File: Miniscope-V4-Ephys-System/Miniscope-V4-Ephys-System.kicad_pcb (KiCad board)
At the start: 4 copper layers, 58.8 x 47 mm, 150 parts, among them J1 34 Circuit Slimslack Connector, J10 Conn_01x01, J11 Conn_01x01, J12 Conn_01x01, J13 Conn_01x01, J14 Conn_01x05, J15 Conn_01x01, J16 Conn_01x01, J17 Conn_01x01, J18 Conn_01x01, J19 Conn_01x01, J2 Conn_01x01, J20 Conn_01x01, J21 Conn_01x01, J22 Conn_01x01, J23 Conn_01x01, J24 Conn_01x01, J25 Conn_01x01, J26 Conn_01x01, J27 Conn_01x01, J28 Conn_01x01, J3 Conn_01x01, J4 Conn_01x01, J5 Conn_01x01, J6 Conn_01x01, J7 Conn_01x01, J8 Conn_01x01, J9 Conn_01x01, Q1 MMBT3904LP-7B, U1 RHD2132, U2 TXB0304RUT, U3 MCP1711T-30I/5X, U4 ATSAME70N21A-CN, U5 MCP1711T-18I/5X, Y1 SMD_CRYSTAL

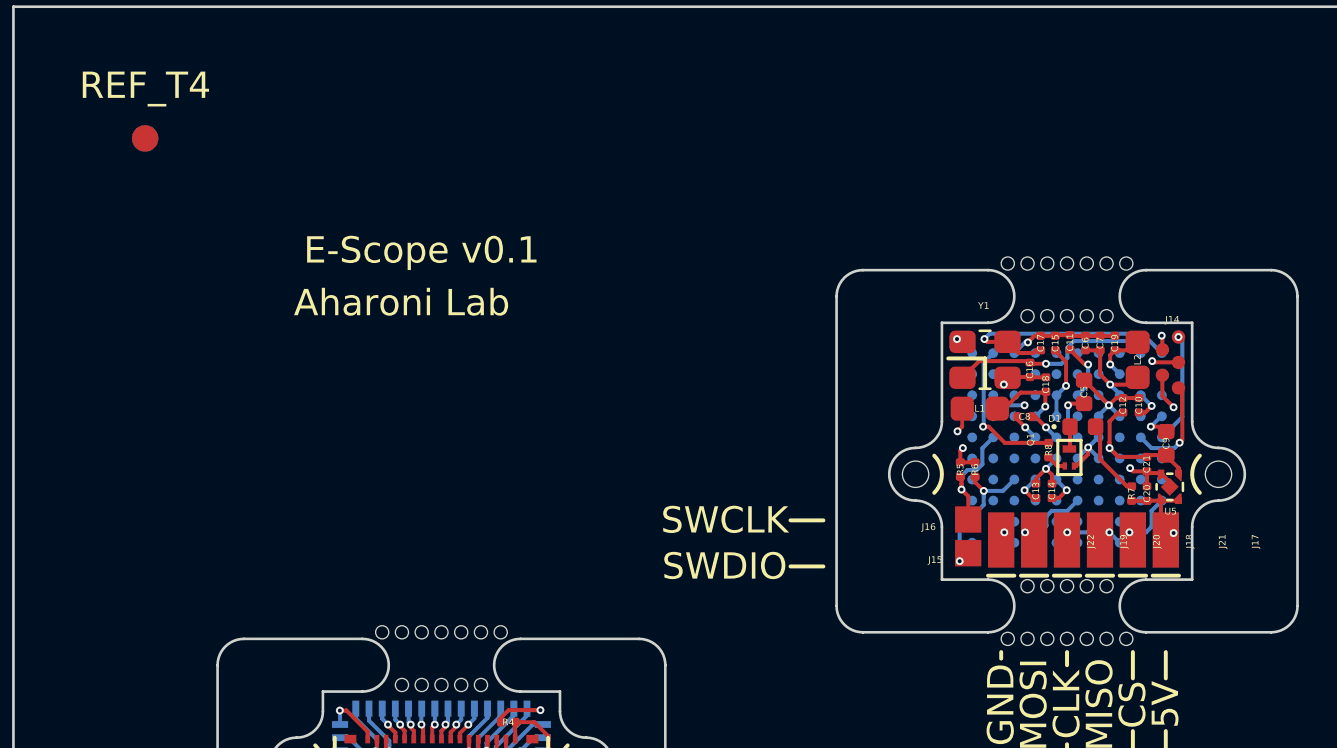
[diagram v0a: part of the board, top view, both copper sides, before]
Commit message: Add files via upload
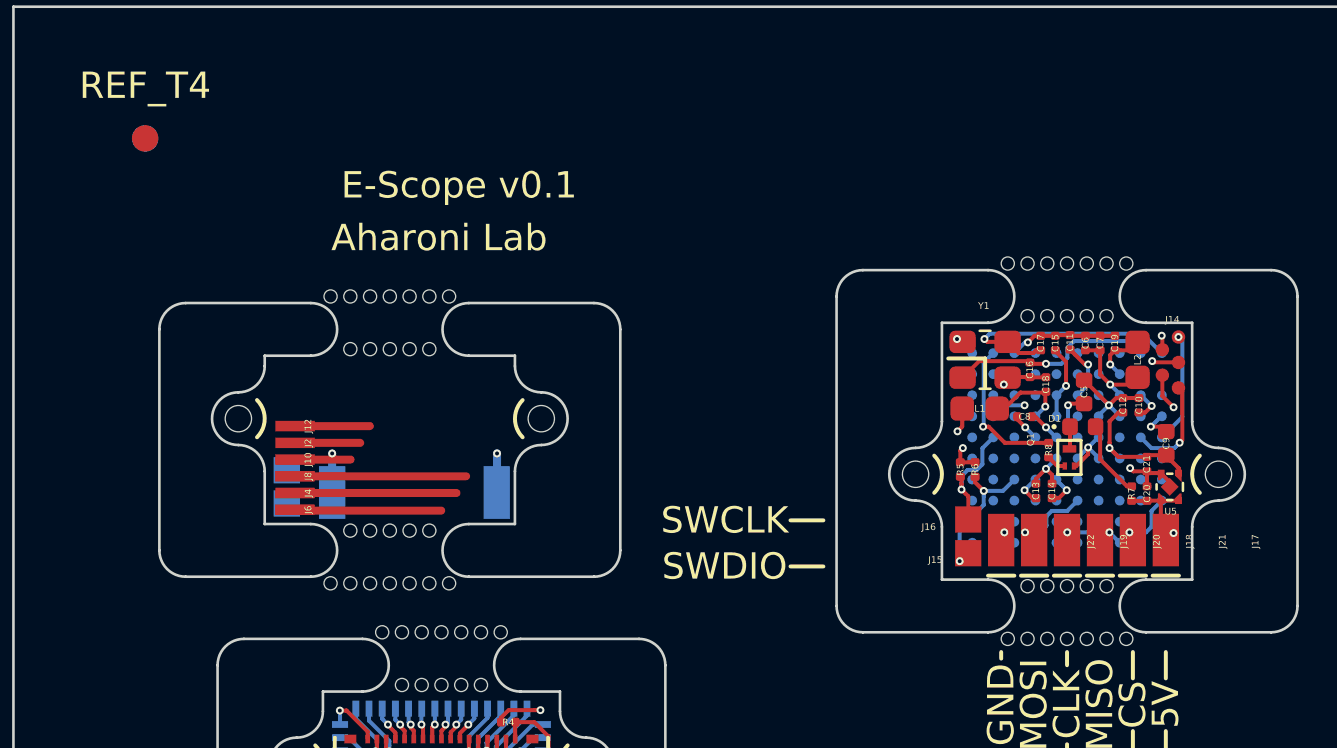
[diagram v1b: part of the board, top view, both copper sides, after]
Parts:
- added HOLE: Conn_1x1_700_Circular_Pad, .Connector:Conn_1x1_700_Circular_Pad, F.Cu at (107.8, 119.9)
- added HOLE: Conn_1x1_700_Circular_Pad, .Connector:Conn_1x1_700_Circular_Pad, F.Cu at (110.8, 111.0)
- added HOLE: Conn_1x1_700_Circular_Pad, .Connector:Conn_1x1_700_Circular_Pad, F.Cu at (110.0, 113.0)
- added HOLE: Conn_1x1_700_Circular_Pad, .Connector:Conn_1x1_700_Circular_Pad, F.Cu at (109.3, 113.0)
- added HOLE: Conn_1x1_700_Circular_Pad, .Connector:Conn_1x1_700_Circular_Pad, F.Cu at (109.3, 111.0)
- added HOLE: Conn_1x1_700_Circular_Pad, .Connector:Conn_1x1_700_Circular_Pad, F.Cu at (107.8, 111.0)
- added HOLE: Conn_1x1_700_Circular_Pad, .Connector:Conn_1x1_700_Circular_Pad, F.Cu at (108.5, 111.0)
- added HOLE: Conn_1x1_700_Circular_Pad, .Connector:Conn_1x1_700_Circular_Pad, F.Cu at (107.8, 113.0)
- added HOLE: Conn_1x1_700_Circular_Pad, .Connector:Conn_1x1_700_Circular_Pad, F.Cu at (110.8, 113.0)
- added HOLE: Conn_1x1_700_Circular_Pad, .Connector:Conn_1x1_700_Circular_Pad, F.Cu at (110.0, 111.0)
- added HOLE: Conn_1x1_700_Circular_Pad, .Connector:Conn_1x1_700_Circular_Pad, F.Cu at (108.5, 113.0)
- added HOLE: Conn_1x1_700_Circular_Pad, .Connector:Conn_1x1_700_Circular_Pad, F.Cu at (108.5, 121.9)
- added HOLE: Conn_1x1_700_Circular_Pad, .Connector:Conn_1x1_700_Circular_Pad, F.Cu at (107.8, 121.9)
- added HOLE: Conn_1x1_700_Circular_Pad, .Connector:Conn_1x1_700_Circular_Pad, F.Cu at (108.5, 119.9)
- added HOLE: Conn_1x1_700_Circular_Pad, .Connector:Conn_1x1_700_Circular_Pad, F.Cu at (109.3, 119.9)
- added HOLE: Conn_1x1_700_Circular_Pad, .Connector:Conn_1x1_700_Circular_Pad, F.Cu at (109.3, 121.9)
- added HOLE: Conn_1x1_700_Circular_Pad, .Connector:Conn_1x1_700_Circular_Pad, F.Cu at (110.8, 121.9)
- added HOLE: Conn_1x1_700_Circular_Pad, .Connector:Conn_1x1_700_Circular_Pad, F.Cu at (110.0, 121.9)
- added HOLE: Conn_1x1_700_Circular_Pad, .Connector:Conn_1x1_700_Circular_Pad, F.Cu at (110.8, 119.9)
- added HOLE: Conn_1x1_700_Circular_Pad, .Connector:Conn_1x1_700_Circular_Pad, F.Cu at (110.0, 119.9)
- added HOLE: Conn_1x1_700_Circular_Pad, .Connector:Conn_1x1_700_Circular_Pad, F.Cu at (107.0, 121.9)
- added HOLE: Conn_1x1_700_Circular_Pad, .Connector:Conn_1x1_700_Circular_Pad, F.Cu at (111.5, 121.9)
- added HOLE: Conn_1x1_700_Circular_Pad, .Connector:Conn_1x1_700_Circular_Pad, F.Cu at (111.5, 111.0)
- added HOLE: Conn_1x1_700_Circular_Pad, .Connector:Conn_1x1_700_Circular_Pad, F.Cu at (107.0, 111.0)
- added HOLE: Conn_1x1_700_Circular_Pad, .Connector:Conn_1x1_700_Circular_Pad, F.Cu at (103.5, 115.6)
- added HOLE: Conn_1x1_700_Circular_Pad, .Connector:Conn_1x1_700_Circular_Pad, F.Cu at (115.0, 115.6)
- added J10: Conn_01x01, .Connector:Conn_1x1_250x750_Pad, F.Cu at (105.7, 117.2)
- added J12: Conn_01x01, .Connector:Conn_1x1_250x750_Pad, F.Cu at (105.7, 115.9)
- added J13: Conn_01x01, .Connector:Conn_1x1_250x750_Pad, B.Cu at (113.3, 118.4)
- added J2: Conn_01x01, .Connector:Conn_1x1_250x750_Pad, F.Cu at (105.7, 116.6)
- added J3: Conn_01x01, .Connector:Conn_1x1_250x750_Pad, B.Cu at (105.4, 118.9)
- added J3: Conn_01x01, .Connector:Conn_1x1_250x750_Pad, B.Cu at (105.4, 117.6)
- added J3: Conn_01x01, .Connector:Conn_1x1_250x750_Pad, B.Cu at (107.1, 118.4)
- added J4: Conn_01x01, .Connector:Conn_1x1_250x750_Pad, F.Cu at (105.7, 118.5)
- added J6: Conn_01x01, .Connector:Conn_1x1_250x750_Pad, F.Cu at (105.7, 119.1)
- added J8: Conn_01x01, .Connector:Conn_1x1_250x750_Pad, F.Cu at (105.7, 117.8)
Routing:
- net (no net): track 0.00 -> 28.6 mm, vias 0 -> 2
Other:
- outline, holes or cut-outs redrawn
